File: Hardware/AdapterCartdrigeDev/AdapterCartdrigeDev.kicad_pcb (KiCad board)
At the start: 2 copper layers, 41.5 x 55.5 mm, 4 parts, among them J1 ROM, U1 28C256

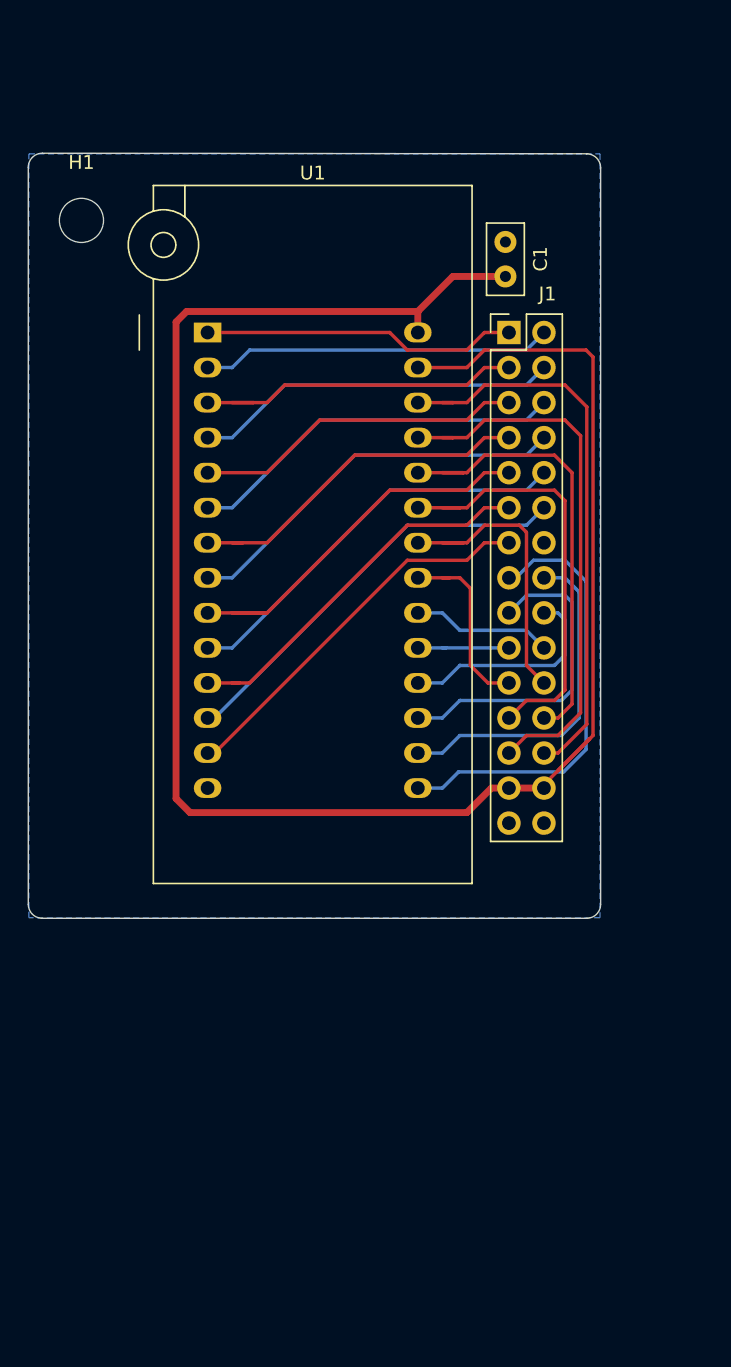
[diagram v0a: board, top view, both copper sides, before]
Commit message: Fix
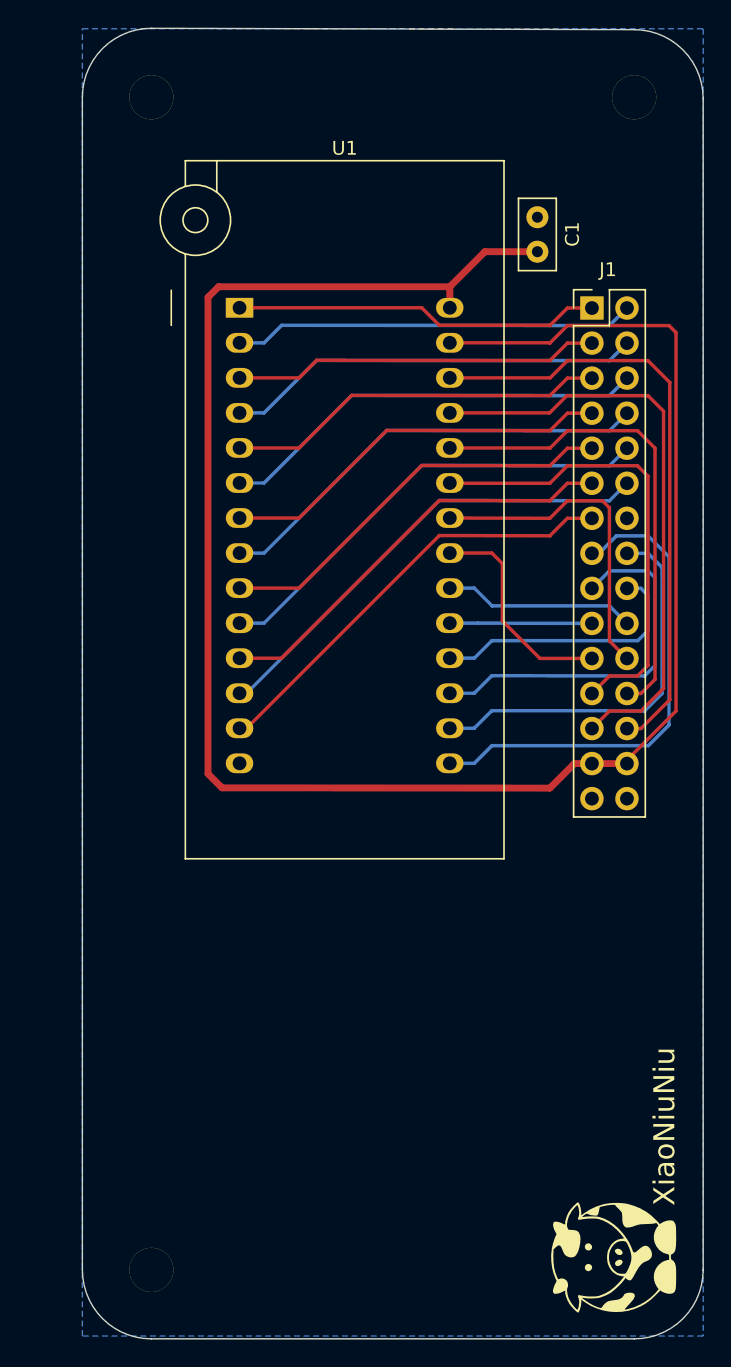
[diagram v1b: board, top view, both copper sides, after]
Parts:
- added H2: MountingHole_Pad, MountingHole:MountingHole_3.2mm_M3, F.Cu at (96.0, 119.0)
- added H3: MountingHole_Pad, MountingHole:MountingHole_3.2mm_M3, F.Cu at (131.0, 34.0)
- added XiaoNiuNiu: LOGO, Logos:VerySmallCow, F.Cu at (129.5, 118.1)
- moved H1 10.3 mm to (96.0, 34.0)
- moved J1 6.27 mm to (127.9, 49.3)
- moved C1 2.93 mm to (124.0, 45.2)
- moved U1 2.93 mm to (102.4, 49.3)
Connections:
- H1 pad : (no net) -> GND
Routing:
- net +5V: track 138.5 -> 142.4 mm
- net CS: track 10.2 -> 13.9 mm
- net /A14: track 22.9 -> 26.6 mm
- net /D4: track 24.8 -> 28.5 mm
- net /D5: track 23.7 -> 27.4 mm
- net /A0: track 29.6 -> 33.3 mm
- net /A5: track 23.9 -> 27.6 mm
- net /A2: track 28.6 -> 32.3 mm
- net /A4: track 27.5 -> 31.2 mm
- net /A6: track 26.5 -> 30.2 mm
- net /A12: track 25.4 -> 29.1 mm
- net /D6: track 15.8 -> 19.5 mm
- net /D7: track 6.86 -> 10.3 mm
- net /D0: track 27.6 -> 30.8 mm
- net /D2: track 28.2 -> 31.3 mm
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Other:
- board size 41.5 x 55.5 mm -> 45 x 95 mm
